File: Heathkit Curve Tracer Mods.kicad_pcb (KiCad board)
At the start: 2 copper layers, 38.1 x 38.1 mm, 12 parts, among them J1 Switch, J2 IC6 Jumper, J3 +15, U1 74LS42, U2 74LVC1G04, U3 74LS90, U4 LM7805_TO220

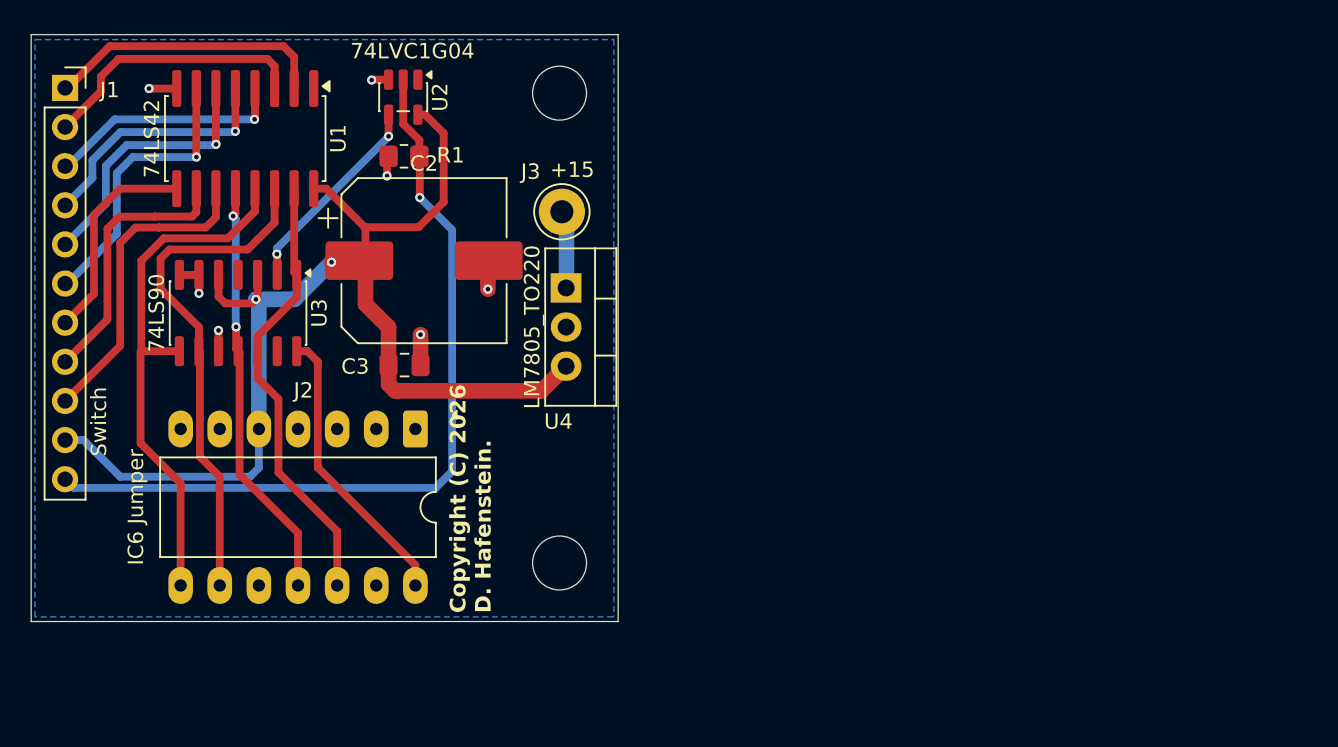
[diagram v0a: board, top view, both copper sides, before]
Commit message: updates
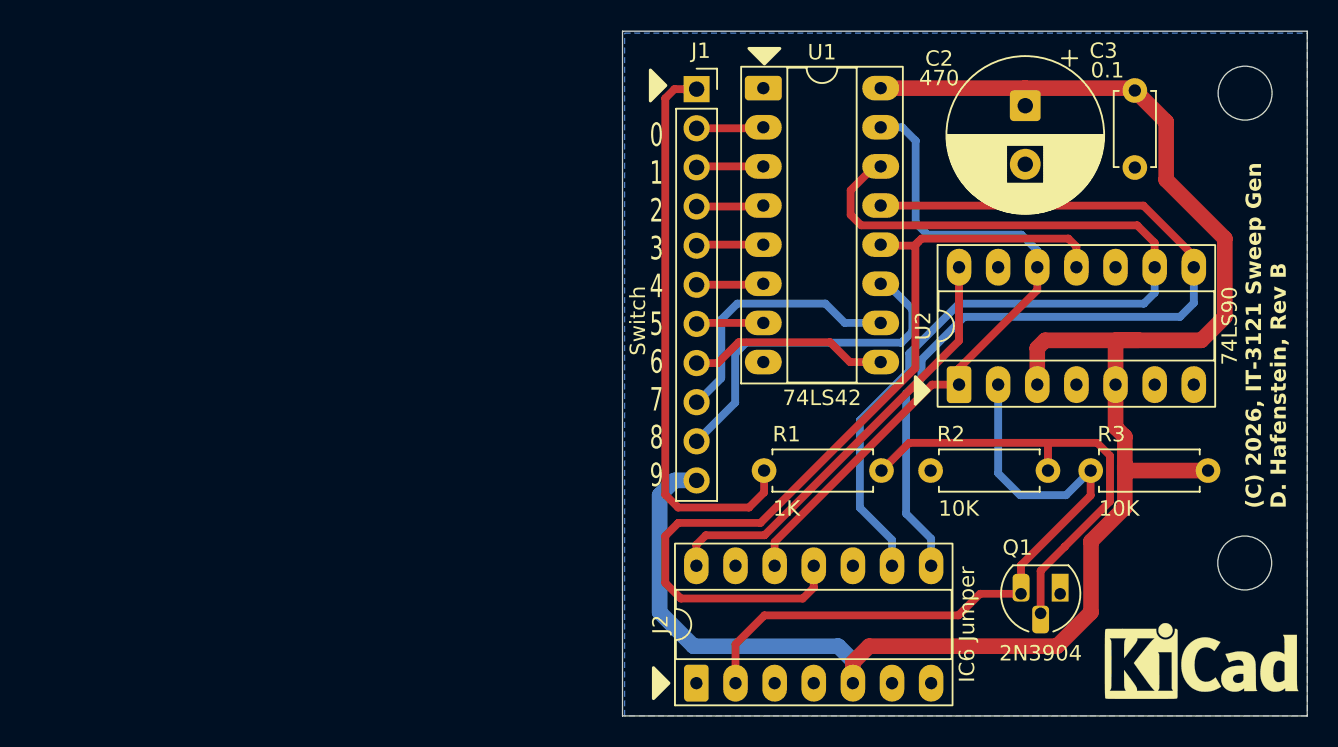
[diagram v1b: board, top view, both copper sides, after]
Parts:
- removed J3: +15, Connector_Pin:Pin_D1.3mm_L11.0mm_LooseFit
- removed U3: 74LS90, Package_SO:SOIC-14_3.9x8.7mm_P1.27mm
- removed U4: LM7805_TO220, Package_TO_SOT_THT:TO-220-3_Vertical
- added Q1: 2N3904, Package_TO_SOT_THT:TO-92L_HandSolder, F.Cu at (106.9, 76.4)
- added R2: 10K, Resistor_THT:R_Axial_DIN0207_L6.3mm_D2.5mm_P7.62mm_Horizontal, F.Cu at (106.1, 68.4)
- added R3: 10K, Resistor_THT:R_Axial_DIN0207_L6.3mm_D2.5mm_P7.62mm_Horizontal, F.Cu at (116.5, 68.4)
- added REF**: KiCad-Logo_5mm_SilkScreen, Symbol:KiCad-Logo_5mm_SilkScreen, F.Cu at (116.1, 81.3)
- C2: footprint Capacitor_SMD:CP_Elec_10x14.3 -> Capacitor_THT:CP_Radial_D10.0mm_P3.80mm
- C3: footprint Capacitor_SMD:C_0805_2012Metric_Pad1.18x1.45mm_HandSolder -> Capacitor_THT:C_Disc_D4.7mm_W2.5mm_P5.00mm
- J2: footprint Package_DIP:DIP-14_W10.16mm_LongPads -> Package_DIP:DIP-14_W7.62mm_Socket_LongPads
- R1: value 10K -> 1K; footprint Resistor_SMD:R_0805_2012Metric_Pad1.20x1.40mm_HandSolder -> Resistor_THT:R_Axial_DIN0207_L6.3mm_D2.5mm_P7.62mm_Horizontal
- U1: footprint Package_SO:SOIC-16W_5.3x10.2mm_P1.27mm -> Package_DIP:DIP-16_W7.62mm_Socket_LongPads
- U2: value 74LVC1G04 -> 74LS90; footprint Package_TO_SOT_SMD:SOT-23-5 -> Package_DIP:DIP-14_W7.62mm_Socket_LongPads
- moved C3 50.6 mm to (111.7, 43.7), turned to -90 degrees
- moved REF** 44.5 mm to (118.9, 43.9)
- moved REF** 44.5 mm to (118.9, 74.4)
- moved J1 41.0 mm to (83.3, 43.6)
- moved U2 40.6 mm to (100.3, 62.8), turned to 90 degrees
- moved C2 40.3 mm to (104.6, 44.7), turned to -90 degrees
- moved U1 33.8 mm to (87.6, 43.6), turned to 0 degrees
- moved R1 31.0 mm to (87.7, 68.4), turned to 0 degrees
- moved J2 24.6 mm to (83.3, 82.2), turned to 90 degrees
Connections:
- J1 pad 10: +5V -> Net-(J1-Pin_10)
- J1 pad 11: Net-(J1-Pin_11) -> +5V
- J2 pad 2: unconnected-(J2-Pin_2-Pad2) -> Net-(J2-Pin_2)
- J2 pad 6: unconnected-(J2-Pin_6-Pad6) -> GND
- R1 pad 1: Net-(J1-Pin_11) -> Net-(J1-Pin_1)
- R1 pad 2: GND -> Net-(Q1-B)
- U1 pad 10: Net-(J1-Pin_8) -> Net-(J1-Pin_9)
- U1 pad 11: Net-(J1-Pin_9) -> Net-(J1-Pin_10)
- U1 pad 2: Net-(J1-Pin_1) -> Net-(J1-Pin_2)
- U1 pad 3: Net-(J1-Pin_2) -> Net-(J1-Pin_3)
- U1 pad 4: Net-(J1-Pin_3) -> Net-(J1-Pin_4)
- U1 pad 5: Net-(J1-Pin_4) -> Net-(J1-Pin_5)
- U1 pad 6: Net-(J1-Pin_5) -> Net-(J1-Pin_6)
- U1 pad 7: Net-(J1-Pin_6) -> Net-(J1-Pin_7)
- U1 pad 9: Net-(J1-Pin_7) -> Net-(J1-Pin_8)
- U2 pad 1: unconnected-(U2-NC-Pad1) -> Net-(J2-Pin_12)
- U2 pad 2: Net-(J1-Pin_11) -> Net-(J2-Pin_2)
- U2 pad 3: GND -> +5V
- U2 pad 4: Net-(U3-R0(1)) -> (no net)
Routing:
- net Net-(J1-Pin_11): track 52.5 -> 0.00 mm, vias 1 -> 0
- net Net-(J2-Pin_2): track 0.00 -> 45.3 mm
- net +5V: track 78.6 -> 120.0 mm, vias 2 -> 0
- net Net-(Q1-B): track 0.00 -> 29.8 mm
- net Net-(J2-Pin_11): track 27.6 -> 56.9 mm, vias 2 -> 0
- net Net-(J2-Pin_9): track 33.4 -> 61.1 mm
- net Net-(J2-Pin_8): track 34.8 -> 57.7 mm
- net Net-(J1-Pin_10): track 0.00 -> 22.6 mm
- net Net-(J1-Pin_1): track 18.1 -> 36.6 mm
- net Net-(J2-Pin_12): track 29.0 -> 45.2 mm
- net Net-(J1-Pin_6): track 18.6 -> 4.27 mm, vias 1 -> 0
- net Net-(U3-R0(1)): track 13.4 -> 0.00 mm, vias 2 -> 0
- net Net-(J1-Pin_2): track 17.6 -> 4.27 mm
- net Net-(J1-Pin_5): track 17.6 -> 4.27 mm, vias 1 -> 0
- net Net-(J1-Pin_4): track 16.5 -> 4.27 mm, vias 1 -> 0
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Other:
- board size 38.1 x 38.1 mm -> 44.5 x 44.5 mm
- board text added: "(C) 2026, IT-3121 Sweep Gen D. Hafenstein, Rev B"
- board text added: "0 1 2 3 4 5 6 7 8 9"
- board text removed: "Copyright (C) 2026 D. Hafenstein."
